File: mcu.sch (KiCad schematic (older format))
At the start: 18 parts, among them SW501 EVQQ2, SW502 EVQQ2, U501 STM32F405RGTx, Y501 8MHz

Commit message: updated part info
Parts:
- C509: MFN (none) -> Murata; MFP (none) -> GRM188R61A105KA61J
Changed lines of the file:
@@
 F 1 "Serial / Bootloader" H 1300 5500 50  0000 C CNN
 F 2 "Pin_Headers:Pin_Header_Straight_1x06_Pitch2.54mm" H 1300 5900 50  0001 C CNN
-F 3 "" H 1300 5900 50  0001 C CNN
+F 3 "http://datasheet.octopart.com/68002-106HLF-FCI-datasheet-8449737.pdf" H 1300 5900 50  0001 C CNN
 F 4 "FCI" H 1300 6300 50  0001 C CNN "MFN"
 F 5 "68002-106HLF" H 1300 6300 50  0001 C CNN "MFP"
@@
 F 1 "JTAG" H 2850 5500 50  0000 C CNN
 F 2 "Pin_Headers:Pin_Header_Straight_2x05_Pitch1.27mm" H 2800 5800 50  0001 C CNN
-F 3 "" H 2800 5800 50  0001 C CNN
+F 3 "http://datasheet.octopart.com/20021111-00010T4LF-FCI-datasheet-11548804.pdf" H 2800 5800 50  0001 C CNN
 F 4 "FCI" H 2850 6200 50  0001 C CNN "MFN"
 F 5 "20021111-00010T4LF" H 2850 6200 50  0001 C CNN "MFP"
@@
 F 1 "1u" H 4025 7050 50  0000 L CNN
 F 2 "Capacitors_SMD:C_0603" H 4038 7000 50  0001 C CNN
-F 3 "" H 4000 7150 50  0001 C CNN
+F 3 "http://datasheet.octopart.com/GRM188R61A105KA61J-Murata-datasheet-66077091.pdf" H 4000 7150 50  0001 C CNN
+F 4 "Murata" H 4025 7350 50  0001 C CNN "MFN"
+F 5 "GRM188R61A105KA61J" H 4025 7350 50  0001 C CNN "MFP"
 	1    4000 7150
 	1    0    0    -1
@@
 F 5 "GRM188R71E104JA01J" H 4325 7350 50  0001 C CNN "MFP"
 	1    4300 7150
+	1    0    0    -1
+$EndComp
+$Comp
+L PWR_FLAG #FLG066
+U 1 1 59F48B1D
+P 1400 2300
+F 0 "#FLG066" H 1400 2375 50  0001 C CNN
+F 1 "PWR_FLAG" H 1400 2450 50  0001 C CNN
+F 2 "" H 1400 2300 50  0001 C CNN
+F 3 "" H 1400 2300 50  0001 C CNN
+	1    1400 2300
+	-1   0    0    1
+$EndComp
+$Comp
+L PWR_FLAG #FLG067
+U 1 1 59F48C86
+P 1400 2000
+F 0 "#FLG067" H 1400 2075 50  0001 C CNN
+F 1 "PWR_FLAG" H 1400 2150 50  0001 C CNN
+F 2 "" H 1400 2000 50  0001 C CNN
+F 3 "" H 1400 2000 50  0001 C CNN
+	1    1400 2000
 	1    0    0    -1
 $EndComp
@@
 Text GLabel 10200 2800 2    51   Output ~ 0
 USB_D+
+Text GLabel 10200 3300 2    51   Output ~ 0
+DAC_SYNC
 Wire Wire Line
 	1500 6100 1600 6100
@@
 Wire Wire Line
 	10100 4800 10200 4800
+Wire Wire Line
+	1400 3700 1500 3700
+Wire Wire Line
+	1400 3800 1500 3800
+Wire Wire Line
+	10100 3500 10200 3500
+Wire Wire Line
+	10100 4300 10200 4300
+Wire Wire Line
+	10200 4400 10100 4400
+Wire Wire Line
+	10200 2400 10100 2400
+Wire Wire Line
+	1400 4200 1500 4200
 Connection ~ 2500 6000
 Connection ~ 2500 5800
@@
 Connection ~ 4000 6900
 Connection ~ 4000 7400
+Connection ~ 1400 2250
+Connection ~ 1400 2050
 NoConn ~ 1500 5600
 NoConn ~ 1500 5900
@@
 NoConn ~ 2600 5900
 NoConn ~ 1500 2000
-Text GLabel 10200 3300 2    51   Output ~ 0
-DAC_SYNC
-Wire Wire Line
-	1400 3700 1500 3700
-Wire Wire Line
-	1400 3800 1500 3800
-Wire Wire Line
-	10100 3500 10200 3500
-Wire Wire Line
-	10100 4300 10200 4300
 NoConn ~ 1500 3500
 NoConn ~ 1500 4400
-Wire Wire Line
-	10200 4400 10100 4400
-Wire Wire Line
-	10200 2400 10100 2400
-Wire Wire Line
-	1400 4200 1500 4200
-$Comp
-L PWR_FLAG #FLG066
-U 1 1 59F48B1D
-P 1400 2300
-F 0 "#FLG066" H 1400 2375 50  0001 C CNN
-F 1 "PWR_FLAG" H 1400 2450 50  0001 C CNN
-F 2 "" H 1400 2300 50  0001 C CNN
-F 3 "" H 1400 2300 50  0001 C CNN
-	1    1400 2300
-	-1   0    0    1
-$EndComp
-Connection ~ 1400 2250
-$Comp
-L PWR_FLAG #FLG067
-U 1 1 59F48C86
-P 1400 2000
-F 0 "#FLG067" H 1400 2075 50  0001 C CNN
-F 1 "PWR_FLAG" H 1400 2150 50  0001 C CNN
-F 2 "" H 1400 2000 50  0001 C CNN
-F 3 "" H 1400 2000 50  0001 C CNN
-	1    1400 2000
-	1    0    0    -1
-$EndComp
-Connection ~ 1400 2050
 NoConn ~ 10100 4200
 NoConn ~ 10100 4100

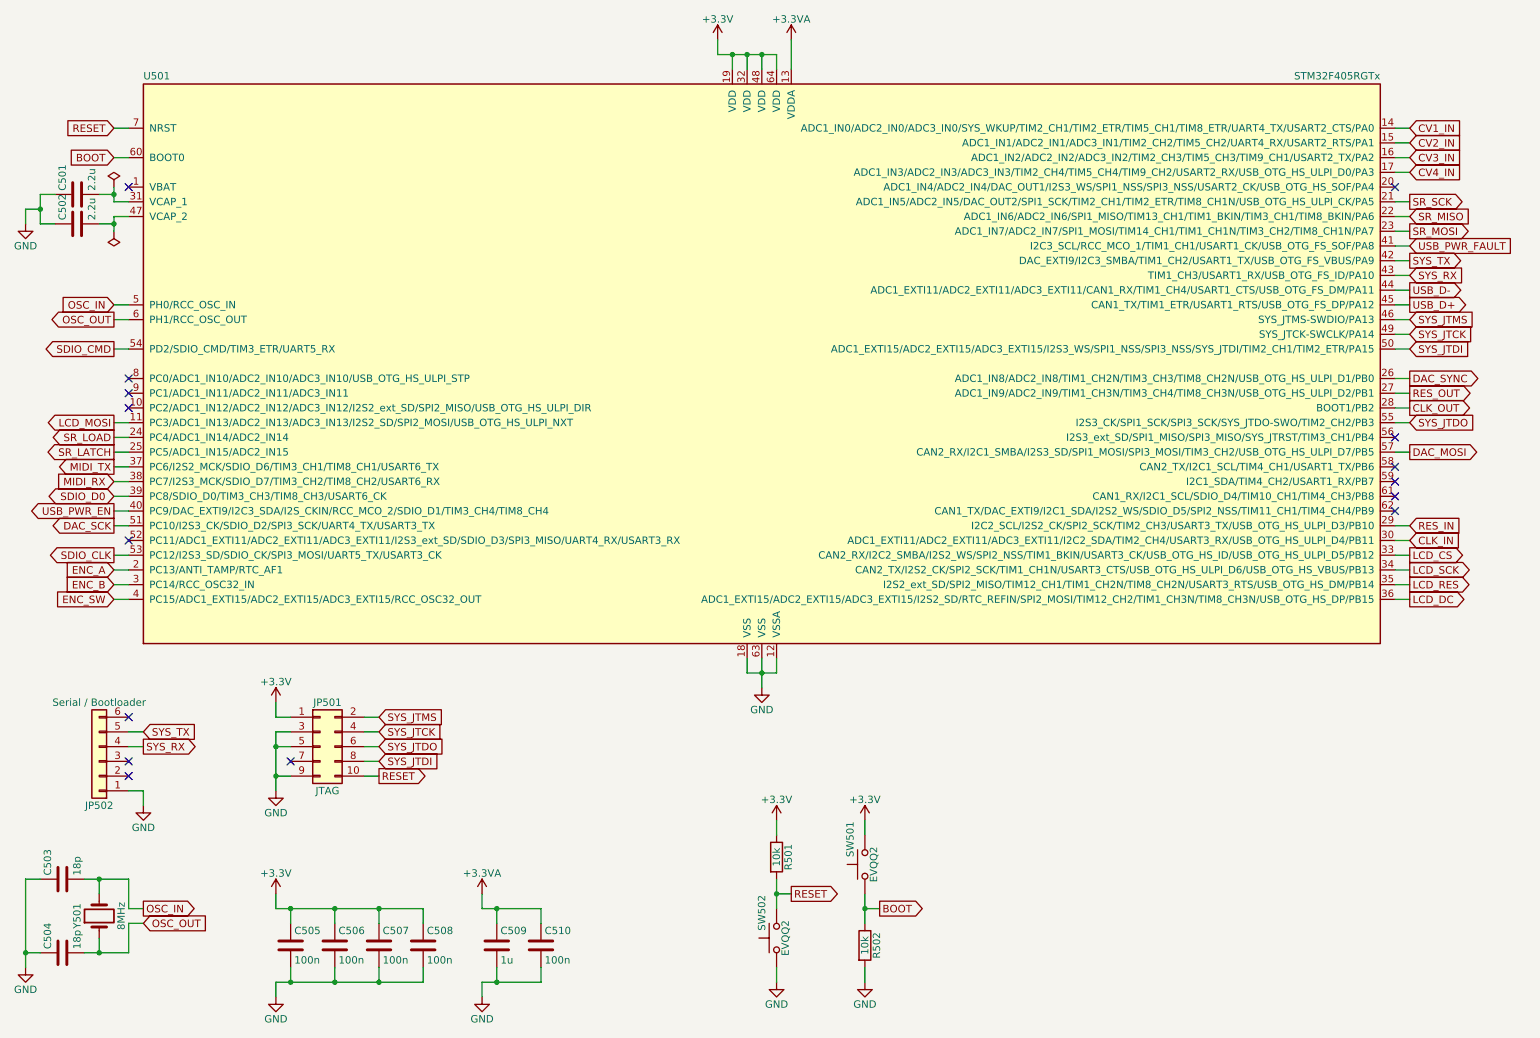
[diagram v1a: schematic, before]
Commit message: work in progress
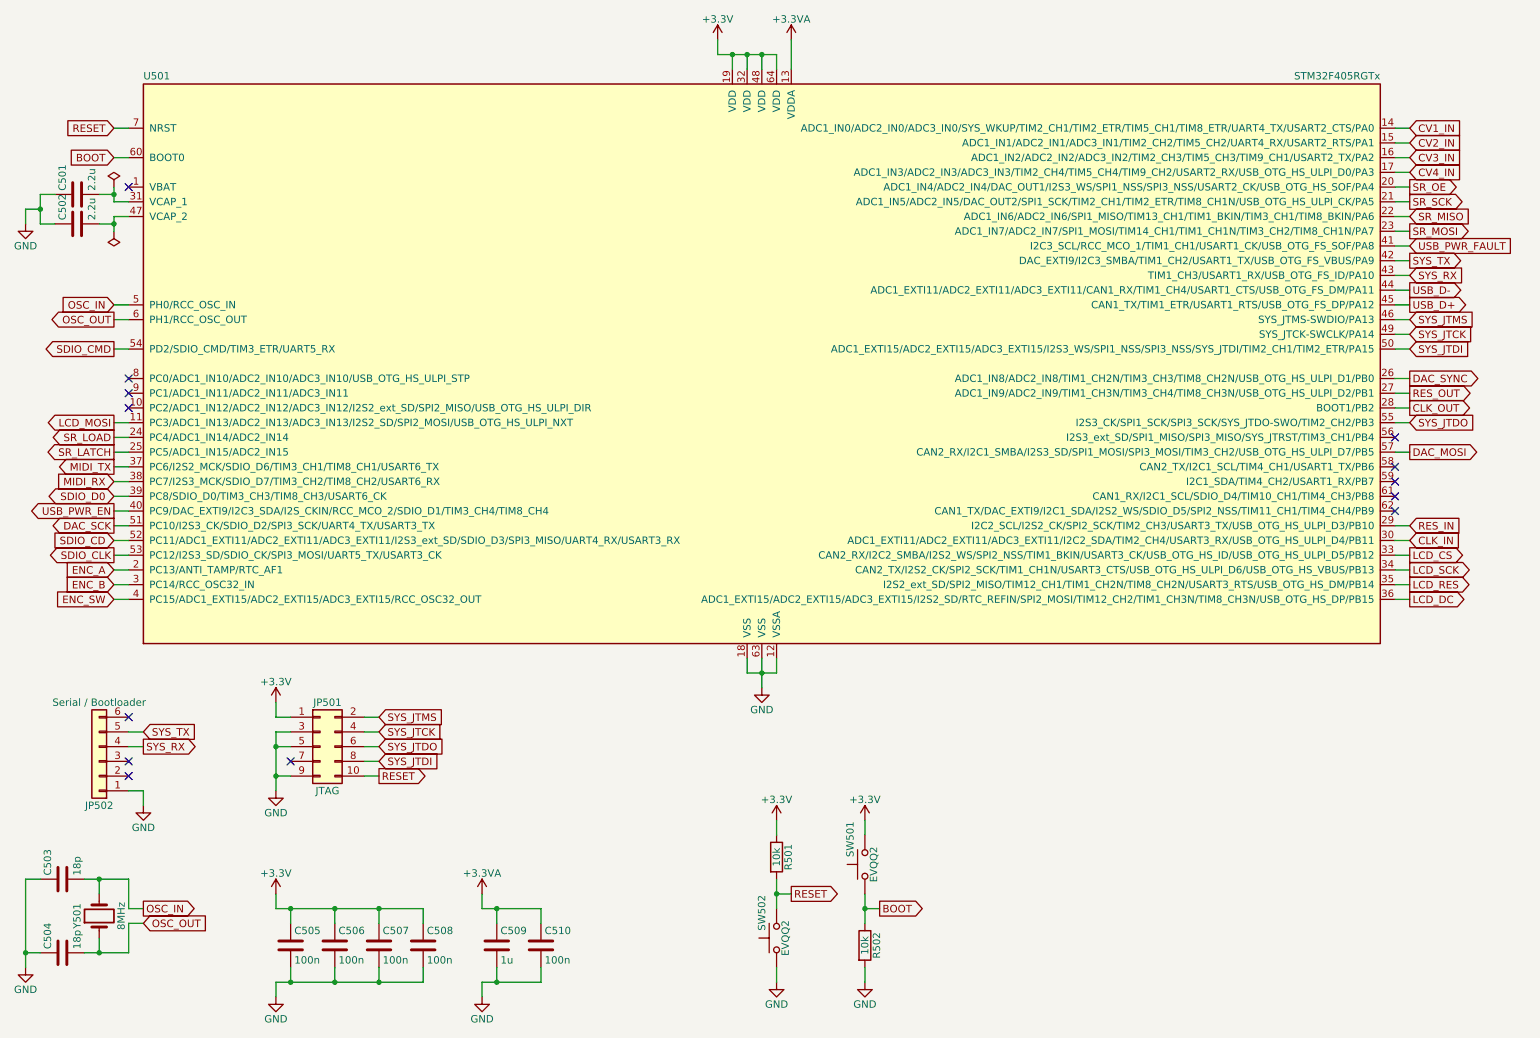
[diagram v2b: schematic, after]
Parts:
- C503, C504, C505, C506, C507, C508, C509, C510: footprint Capacitors_SMD:C_0603 -> Capacitors_SMD:C_0603_HandSoldering
- R501, R502: footprint Resistors_SMD:R_0603 -> Resistors_SMD:R_0603_HandSoldering
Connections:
- net SR_OE: now reaches U501.20 (ADC1_IN4/ADC2_IN4/DAC_OUT1/I2S3_WS/SPI1_NSS/SPI3_NSS/USART2_CK/USB_OTG_HS_SOF/PA4)
- net SDIO_CD: now reaches U501.52 (PC11/ADC1_EXTI11/ADC2_EXTI11/ADC3_EXTI11/I2S3_ext_SD/SDIO_D3/SPI3_MISO/UART4_RX/USART3_RX)
- no-connect marks 15 -> 13
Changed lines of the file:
@@
 $EndComp
 $Comp
-L GND #PWR050
+L GND #PWR052
 U 1 1 59DB9615
 P 1600 6200
-F 0 "#PWR050" H 1600 5950 50  0001 C CNN
+F 0 "#PWR052" H 1600 5950 50  0001 C CNN
 F 1 "GND" H 1600 6050 50  0000 C CNN
 F 2 "" H 1600 6200 50  0001 C CNN
@@
 $EndComp
 $Comp
-L +3.3V #PWR051
+L +3.3V #PWR053
 U 1 1 59DB9CCC
 P 2500 5500
-F 0 "#PWR051" H 2500 5350 50  0001 C CNN
+F 0 "#PWR053" H 2500 5350 50  0001 C CNN
 F 1 "+3.3V" H 2500 5640 50  0000 C CNN
 F 2 "" H 2500 5500 50  0001 C CNN
@@
 $EndComp
 $Comp
-L GND #PWR052
+L GND #PWR054
 U 1 1 59DB9CF4
 P 2500 6100
-F 0 "#PWR052" H 2500 5850 50  0001 C CNN
+F 0 "#PWR054" H 2500 5850 50  0001 C CNN
 F 1 "GND" H 2500 5950 50  0000 C CNN
 F 2 "" H 2500 6100 50  0001 C CNN
@@
 $EndComp
 $Comp
-L +3.3V #PWR053
+L +3.3V #PWR055
 U 1 1 59DB9EAC
 P 5500 1000
-F 0 "#PWR053" H 5500 850 50  0001 C CNN
+F 0 "#PWR055" H 5500 850 50  0001 C CNN
 F 1 "+3.3V" H 5500 1140 50  0000 C CNN
 F 2 "" H 5500 1000 50  0001 C CNN
@@
 $EndComp
 $Comp
-L +3.3VA #PWR054
+L +3.3VA #PWR056
 U 1 1 59DB9EE7
 P 6000 1000
-F 0 "#PWR054" H 6000 850 50  0001 C CNN
+F 0 "#PWR056" H 6000 850 50  0001 C CNN
 F 1 "+3.3VA" H 6000 1140 50  0000 C CNN
 F 2 "" H 6000 1000 50  0001 C CNN
@@
 $EndComp
 $Comp
-L GND #PWR055
+L GND #PWR057
 U 1 1 59DB9FE7
 P 5800 5400
-F 0 "#PWR055" H 5800 5150 50  0001 C CNN
+F 0 "#PWR057" H 5800 5150 50  0001 C CNN
 F 1 "GND" H 5800 5250 50  0000 C CNN
 F 2 "" H 5800 5400 50  0001 C CNN
@@
 F 0 "C503" H 1075 6800 50  0000 L CNN
 F 1 "18p" H 1075 6600 50  0000 L CNN
-F 2 "Capacitors_SMD:C_0603" H 1088 6550 50  0001 C CNN
+F 2 "Capacitors_SMD:C_0603_HandSoldering" H 1088 6550 50  0001 C CNN
 F 3 "http://datasheet.octopart.com/GRM1885C1H180JA01J-Murata-datasheet-66077082.pdf" H 1050 6700 50  0001 C CNN
 F 4 "Murata" H 1075 6900 50  0001 C CNN "MFN"
@@
 F 0 "C504" H 1075 7300 50  0000 L CNN
 F 1 "18p" H 1075 7100 50  0000 L CNN
-F 2 "Capacitors_SMD:C_0603" H 1088 7050 50  0001 C CNN
+F 2 "Capacitors_SMD:C_0603_HandSoldering" H 1088 7050 50  0001 C CNN
 F 3 "http://datasheet.octopart.com/GRM1885C1H180JA01J-Murata-datasheet-66077082.pdf" H 1050 7200 50  0001 C CNN
 F 4 "Murata" H 1075 7400 50  0001 C CNN "MFN"
@@
 $EndComp
 $Comp
-L GND #PWR056
+L GND #PWR058
 U 1 1 59DBA437
 P 800 7300
-F 0 "#PWR056" H 800 7050 50  0001 C CNN
+F 0 "#PWR058" H 800 7050 50  0001 C CNN
 F 1 "GND" H 800 7150 50  0000 C CNN
 F 2 "" H 800 7300 50  0001 C CNN
@@
 $EndComp
 $Comp
-L GND #PWR057
+L GND #PWR059
 U 1 1 59DBB736
 P 800 2250
-F 0 "#PWR057" H 800 2000 50  0001 C CNN
+F 0 "#PWR059" H 800 2000 50  0001 C CNN
 F 1 "GND" H 800 2100 50  0000 C CNN
 F 2 "" H 800 2250 50  0001 C CNN
@@
 F 0 "R501" V 5980 6550 50  0000 C CNN
 F 1 "10k" V 5900 6550 50  0000 C CNN
-F 2 "Resistors_SMD:R_0603" V 5830 6550 50  0001 C CNN
+F 2 "Resistors_SMD:R_0603_HandSoldering" V 5830 6550 50  0001 C CNN
 F 3 "http://datasheet.octopart.com/ERJ-3EKF1002V-Panasonic-datasheet-13266541.pdf" H 5900 6550 50  0001 C CNN
 F 4 "Panasonic" H 5980 6650 50  0001 C CNN "MFN"
@@
 F 0 "R502" V 6580 7150 50  0000 C CNN
 F 1 "10k" V 6500 7150 50  0000 C CNN
-F 2 "Resistors_SMD:R_0603" V 6430 7150 50  0001 C CNN
+F 2 "Resistors_SMD:R_0603_HandSoldering" V 6430 7150 50  0001 C CNN
 F 3 "http://datasheet.octopart.com/ERJ-3EKF1002V-Panasonic-datasheet-13266541.pdf" H 6500 7150 50  0001 C CNN
 F 4 "Panasonic" H 6580 7250 50  0001 C CNN "MFN"
@@
 $EndComp
 $Comp
-L +3.3V #PWR058
+L +3.3V #PWR060
 U 1 1 59DD49A9
 P 5900 6300
-F 0 "#PWR058" H 5900 6150 50  0001 C CNN
+F 0 "#PWR060" H 5900 6150 50  0001 C CNN
 F 1 "+3.3V" H 5900 6440 50  0000 C CNN
 F 2 "" H 5900 6300 50  0001 C CNN
@@
 $EndComp
 $Comp
-L +3.3V #PWR059
+L +3.3V #PWR061
 U 1 1 59DD49E1
 P 6500 6300
-F 0 "#PWR059" H 6500 6150 50  0001 C CNN
+F 0 "#PWR061" H 6500 6150 50  0001 C CNN
 F 1 "+3.3V" H 6500 6440 50  0000 C CNN
 F 2 "" H 6500 6300 50  0001 C CNN
@@
 $EndComp
 $Comp
-L GND #PWR060
+L GND #PWR062
 U 1 1 59DD4A83
 P 5900 7400
-F 0 "#PWR060" H 5900 7150 50  0001 C CNN
+F 0 "#PWR062" H 5900 7150 50  0001 C CNN
 F 1 "GND" H 5900 7250 50  0000 C CNN
 F 2 "" H 5900 7400 50  0001 C CNN
@@
 $EndComp
 $Comp
-L GND #PWR061
+L GND #PWR063
 U 1 1 59DD4ABB
 P 6500 7400
-F 0 "#PWR061" H 6500 7150 50  0001 C CNN
+F 0 "#PWR063" H 6500 7150 50  0001 C CNN
 F 1 "GND" H 6500 7250 50  0000 C CNN
 F 2 "" H 6500 7400 50  0001 C CNN
@@
 F 0 "C505" H 2625 7250 50  0000 L CNN
 F 1 "100n" H 2625 7050 50  0000 L CNN
-F 2 "Capacitors_SMD:C_0603" H 2638 7000 50  0001 C CNN
+F 2 "Capacitors_SMD:C_0603_HandSoldering" H 2638 7000 50  0001 C CNN
 F 3 "http://datasheet.octopart.com/GRM188R71E104JA01J-Murata-datasheet-66077098.pdf" H 2600 7150 50  0001 C CNN
 F 4 "Murata" H 2625 7350 50  0001 C CNN "MFN"
@@
 F 0 "C506" H 2925 7250 50  0000 L CNN
 F 1 "100n" H 2925 7050 50  0000 L CNN
-F 2 "Capacitors_SMD:C_0603" H 2938 7000 50  0001 C CNN
+F 2 "Capacitors_SMD:C_0603_HandSoldering" H 2938 7000 50  0001 C CNN
 F 3 "http://datasheet.octopart.com/GRM188R71E104JA01J-Murata-datasheet-66077098.pdf" H 2900 7150 50  0001 C CNN
 F 4 "Murata" H 2925 7350 50  0001 C CNN "MFN"
@@
 F 0 "C507" H 3225 7250 50  0000 L CNN
 F 1 "100n" H 3225 7050 50  0000 L CNN
-F 2 "Capacitors_SMD:C_0603" H 3238 7000 50  0001 C CNN
+F 2 "Capacitors_SMD:C_0603_HandSoldering" H 3238 7000 50  0001 C CNN
 F 3 "http://datasheet.octopart.com/GRM188R71E104JA01J-Murata-datasheet-66077098.pdf" H 3200 7150 50  0001 C CNN
 F 4 "Murata" H 3225 7350 50  0001 C CNN "MFN"
@@
 F 0 "C508" H 3525 7250 50  0000 L CNN
 F 1 "100n" H 3525 7050 50  0000 L CNN
-F 2 "Capacitors_SMD:C_0603" H 3538 7000 50  0001 C CNN
+F 2 "Capacitors_SMD:C_0603_HandSoldering" H 3538 7000 50  0001 C CNN
 F 3 "http://datasheet.octopart.com/GRM188R71E104JA01J-Murata-datasheet-66077098.pdf" H 3500 7150 50  0001 C CNN
 F 4 "Murata" H 3525 7350 50  0001 C CNN "MFN"
@@
 $EndComp
 $Comp
-L +3.3V #PWR062
+L +3.3V #PWR064
 U 1 1 59E34B90
 P 2500 6800
-F 0 "#PWR062" H 2500 6650 50  0001 C CNN
+F 0 "#PWR064" H 2500 6650 50  0001 C CNN
 F 1 "+3.3V" H 2500 6940 50  0000 C CNN
 F 2 "" H 2500 6800 50  0001 C CNN
@@
 $EndComp
 $Comp
-L GND #PWR063
+L GND #PWR065
 U 1 1 59E34BD4
 P 2500 7500
-F 0 "#PWR063" H 2500 7250 50  0001 C CNN
+F 0 "#PWR065" H 2500 7250 50  0001 C CNN
 F 1 "GND" H 2500 7350 50  0000 C CNN
 F 2 "" H 2500 7500 50  0001 C CNN
@@
 $EndComp
 $Comp
-L +3.3VA #PWR064
+L +3.3VA #PWR066
 U 1 1 59E35078
 P 3900 6800
-F 0 "#PWR064" H 3900 6650 50  0001 C CNN
+F 0 "#PWR066" H 3900 6650 50  0001 C CNN
 F 1 "+3.3VA" H 3900 6940 50  0000 C CNN
 F 2 "" H 3900 6800 50  0001 C CNN
@@
 $EndComp
 $Comp
-L GND #PWR065
+L GND #PWR067
 U 1 1 59E350BC
 P 3900 7500
-F 0 "#PWR065" H 3900 7250 50  0001 C CNN
+F 0 "#PWR067" H 3900 7250 50  0001 C CNN
 F 1 "GND" H 3900 7350 50  0000 C CNN
 F 2 "" H 3900 7500 50  0001 C CNN
@@
 F 0 "C509" H 4025 7250 50  0000 L CNN
 F 1 "1u" H 4025 7050 50  0000 L CNN
-F 2 "Capacitors_SMD:C_0603" H 4038 7000 50  0001 C CNN
+F 2 "Capacitors_SMD:C_0603_HandSoldering" H 4038 7000 50  0001 C CNN
 F 3 "http://datasheet.octopart.com/GRM188R61A105KA61J-Murata-datasheet-66077091.pdf" H 4000 7150 50  0001 C CNN
 F 4 "Murata" H 4025 7350 50  0001 C CNN "MFN"
@@
 F 0 "C510" H 4325 7250 50  0000 L CNN
 F 1 "100n" H 4325 7050 50  0000 L CNN
-F 2 "Capacitors_SMD:C_0603" H 4338 7000 50  0001 C CNN
+F 2 "Capacitors_SMD:C_0603_HandSoldering" H 4338 7000 50  0001 C CNN
 F 3 "http://datasheet.octopart.com/GRM188R71E104JA01J-Murata-datasheet-66077098.pdf" H 4300 7150 50  0001 C CNN
 F 4 "Murata" H 4325 7350 50  0001 C CNN "MFN"
@@
 $EndComp
 $Comp
-L PWR_FLAG #FLG066
+L PWR_FLAG #FLG068
 U 1 1 59F48B1D
 P 1400 2300
-F 0 "#FLG066" H 1400 2375 50  0001 C CNN
+F 0 "#FLG068" H 1400 2375 50  0001 C CNN
 F 1 "PWR_FLAG" H 1400 2450 50  0001 C CNN
 F 2 "" H 1400 2300 50  0001 C CNN
@@
 $EndComp
 $Comp
-L PWR_FLAG #FLG067
+L PWR_FLAG #FLG069
 U 1 1 59F48C86
 P 1400 2000
-F 0 "#FLG067" H 1400 2075 50  0001 C CNN
+F 0 "#FLG069" H 1400 2075 50  0001 C CNN
 F 1 "PWR_FLAG" H 1400 2150 50  0001 C CNN
 F 2 "" H 1400 2000 50  0001 C CNN
@@
 NoConn ~ 1500 2000
 NoConn ~ 1500 3500
-NoConn ~ 1500 4400
 NoConn ~ 10100 4200
 NoConn ~ 10100 4100
@@
 NoConn ~ 10100 3900
 NoConn ~ 10100 3700
-NoConn ~ 10100 2000
 NoConn ~ 1500 3300
 NoConn ~ 1500 3400
+Text GLabel 1400 4400 0    51   Input ~ 0
+SDIO_CD
+Wire Wire Line
+	1400 4400 1500 4400
+Text GLabel 10200 2000 2    51   Output ~ 0
+SR_OE
+Wire Wire Line
+	10100 2000 10200 2000
 $EndSCHEMATC
